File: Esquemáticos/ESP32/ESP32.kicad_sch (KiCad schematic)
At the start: 1 part

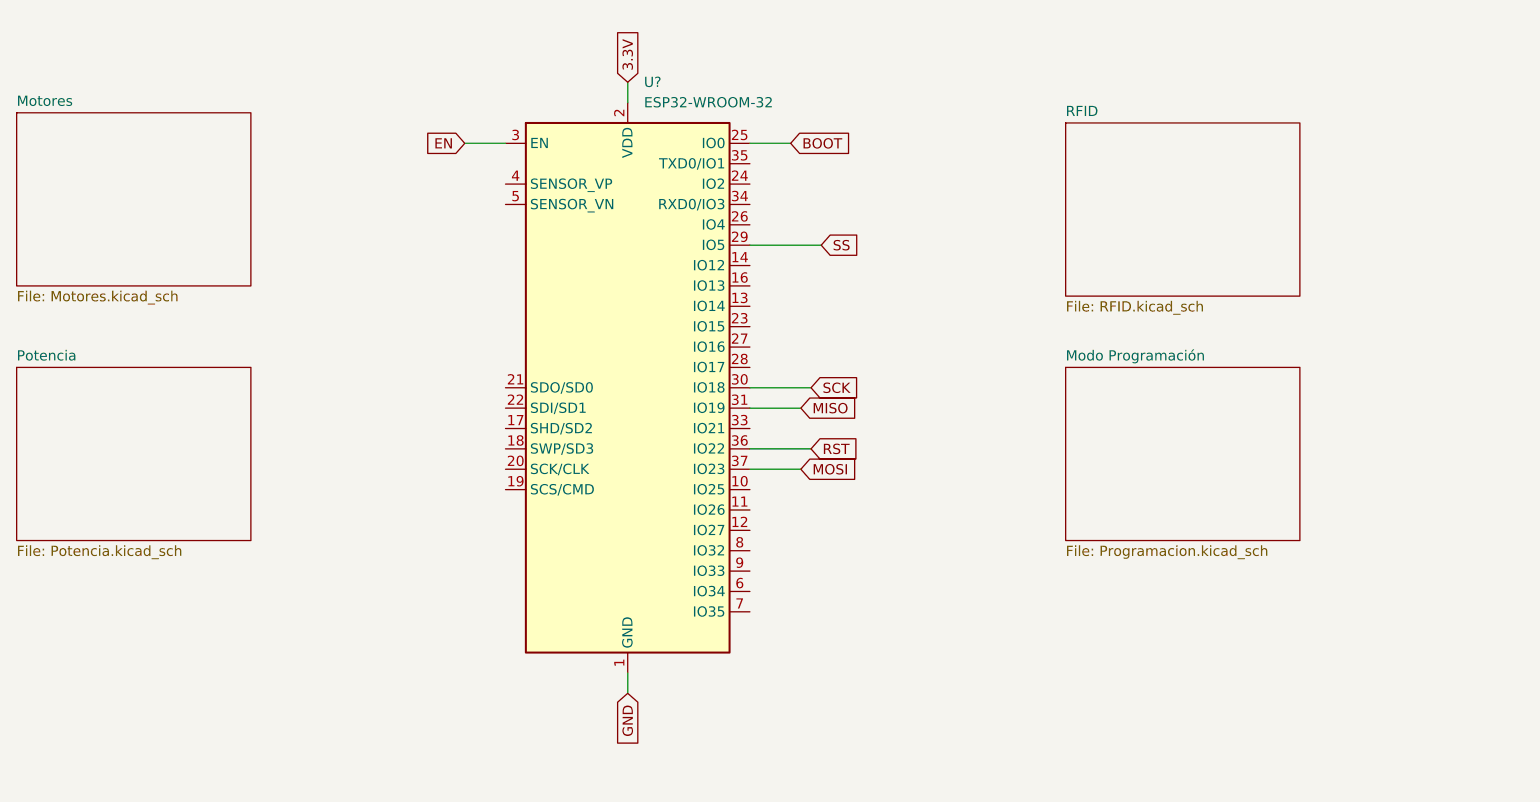
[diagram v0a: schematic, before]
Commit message: Cambios hechos al esquemático, faltan detalles
Revisar el discord para dejar todo al día con el feedback de hoy
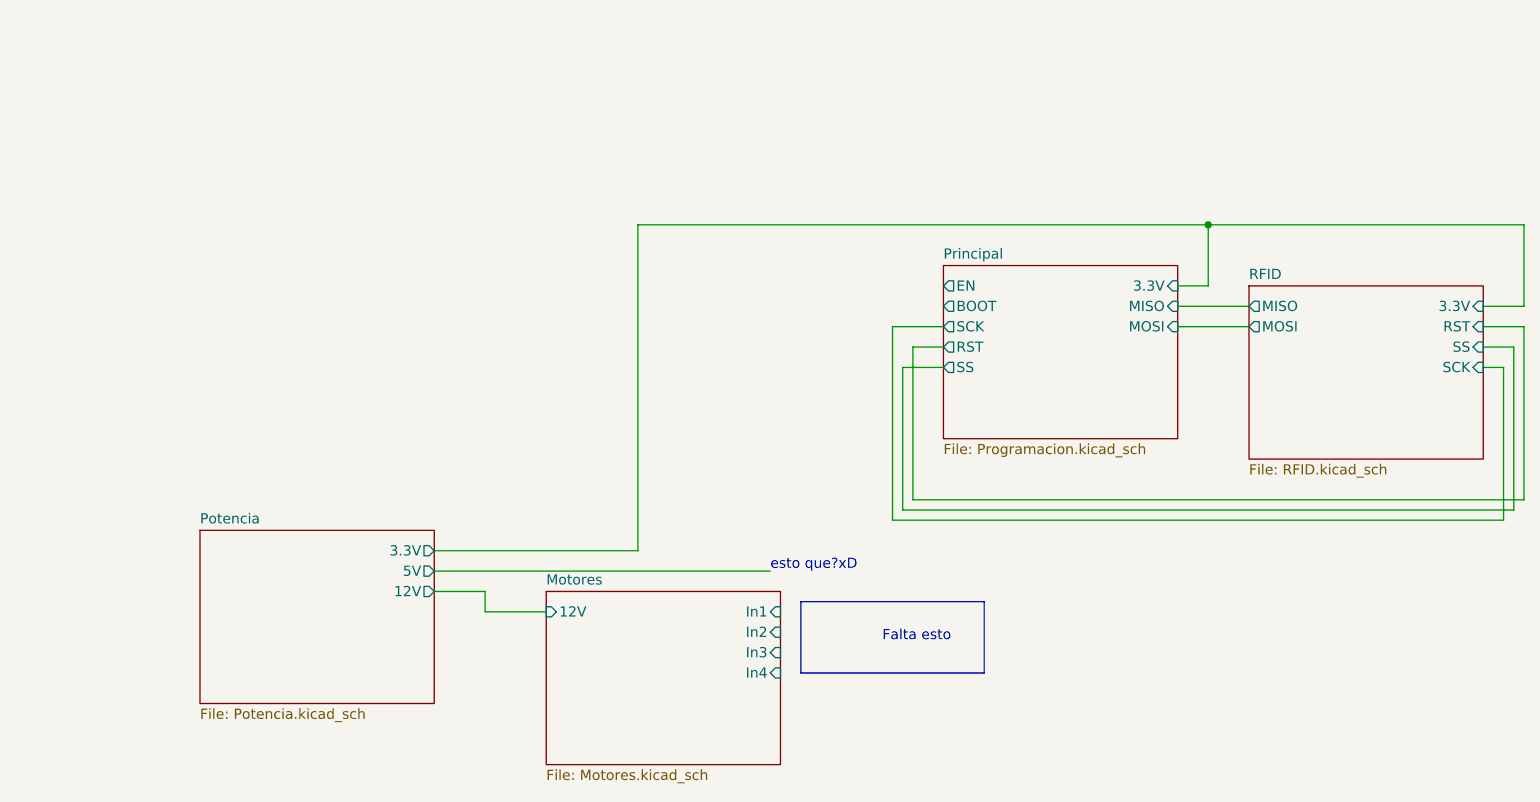
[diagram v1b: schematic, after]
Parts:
- removed U?: ESP32-WROOM-32, RF_Module:ESP32-WROOM-32, symbol RF_Module:ESP32-WROOM-32
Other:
- sheet Modo Programación renamed Principal
- sheet Motores ports: added 12V, In1, In2, In3, In4; removed none
- sheet Potencia ports: added 12V, 3.3V, 5V; removed none
- sheet Principal ports: added 3.3V, BOOT, EN, MISO, MOSI, RST, SCK, SS; removed none
- sheet RFID ports: added 3.3V, MISO, MOSI, RST, SCK, SS; removed none
- note added: "Falta esto"
- note added: "esto que?xD"
